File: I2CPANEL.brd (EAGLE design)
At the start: 54 x 83 mm, 47 parts, among them IC1 ATMEGA32U4-QFN

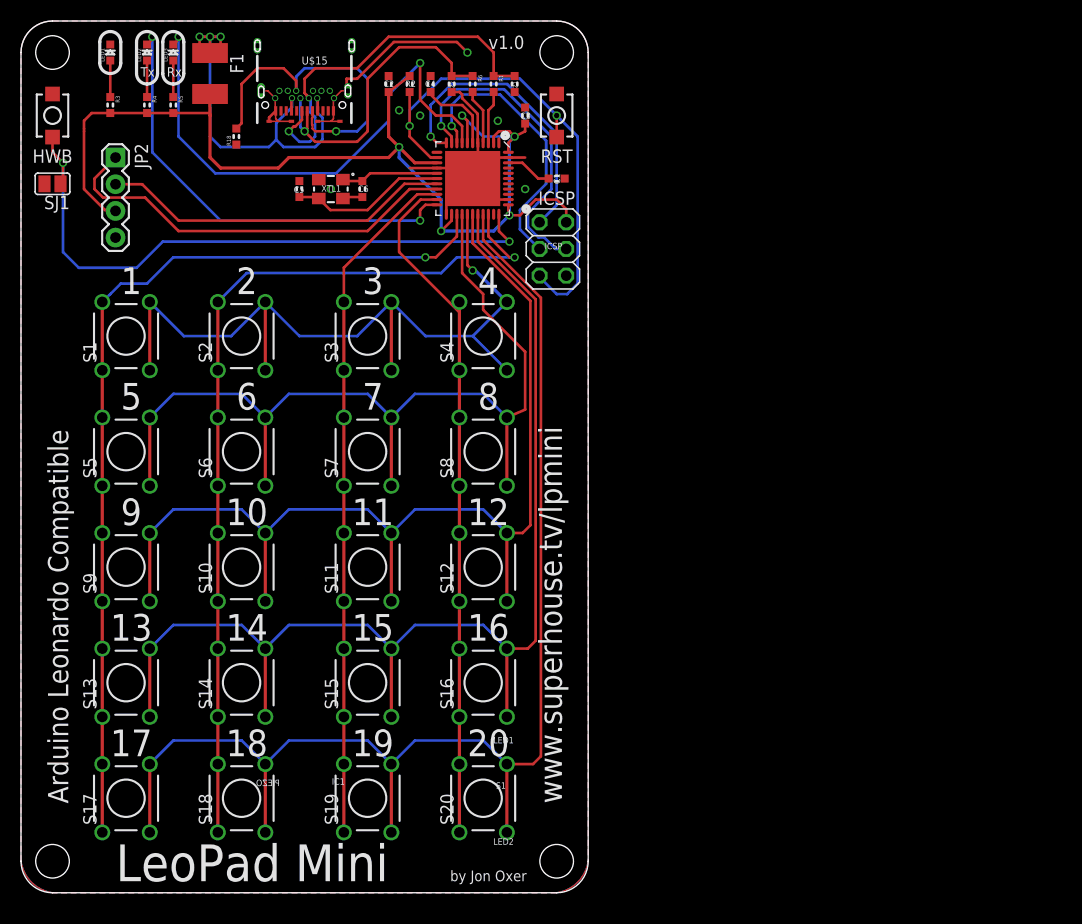
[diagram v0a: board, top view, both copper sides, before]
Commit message: Schematic and routing for v1.0 release
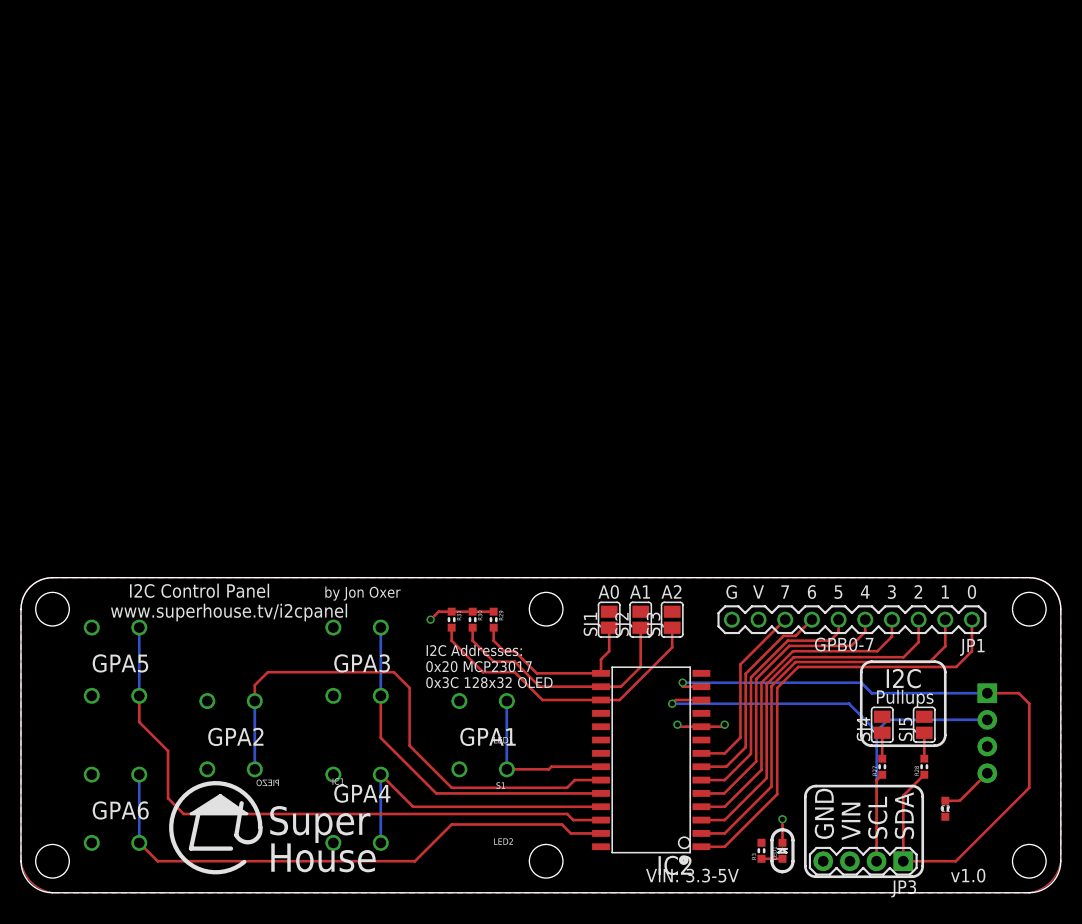
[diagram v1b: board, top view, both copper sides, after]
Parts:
- removed C1: 100nF 0603, freetronics-master-v1.1:0603
- removed C3, C4: 1uF 0603, freetronics-master-v1.1:0603
- removed C5, C6: 15pF 0603, freetronics-master-v1.1:0603
- removed F1: 500mA PTC 1812, rcl:L1812
- removed IC1: ATMEGA32U4-QFN, freetronics-jon:QFN-44N
- removed ICSP: ICSP, pinhead:2X03
- removed LED2: RED, freetronics-jon:LED-0603
- removed LED3: GREEN, freetronics-jon:LED-0603
- removed R1, R6: 22R, freetronics-jon:0603
- removed R18: 5.1K, freetronics-original:0603
- removed R2: 10K 0603, freetronics-master-v1.1:0603
- removed R4, R5: 1K, freetronics-jon:0603
- removed S10: 10, freetronics-original:TACTILE-PTH
- removed S11: 11, freetronics-original:TACTILE-PTH
- removed S12: 12, freetronics-original:TACTILE-PTH
- removed S13: 13, freetronics-original:TACTILE-PTH
- removed S14: 14, freetronics-original:TACTILE-PTH
- removed S15: 15, freetronics-original:TACTILE-PTH
- removed S16: 16, freetronics-original:TACTILE-PTH
- removed S17: 17, freetronics-original:TACTILE-PTH
- removed S18: 18, freetronics-original:TACTILE-PTH
- removed S19: 19, freetronics-original:TACTILE-PTH
- removed S20: 20, freetronics-original:TACTILE-PTH
- removed S21: RESET, freetronics-jon:TACTILE_SWITCH_SMD_2PIN_TINY
- removed S22: HWB, freetronics-jon:TACTILE_SWITCH_SMD_2PIN_TINY
- removed S7: 7, freetronics-original:TACTILE-PTH
- removed S8: 8, freetronics-original:TACTILE-PTH
- removed S9: 9, freetronics-original:TACTILE-PTH
- removed U$15: USB-C, freetronics-jon:USB-C-U52A
- removed XTL1: 16MHz, freetronics-jon:CRYSTAL-SMD-3X2
- removed Z1, Z2: PGB1010603, freetronics-master-v1.1:0603
- added IC2: MCP23017SO, microchip:SO28W
- added JP1: M100.1, freetronics-original:1X10
- added JP3: OLED, freetronics-jon:1X04
- added R27, R28: 4K7, freetronics-master-v1:0603
- added R29, R30, R31: 10K, freetronics-master-v1:0603
- added SJ2, SJ3, SJ4, SJ5: (no value), freetronics-jon:SJ
- C2: value 100nF 0603 -> 1uF
- SJ1: value HWB -> (none)
- moved LED1 99.4 mm to (72.5, 4.00)
- moved JP2 97.4 mm to (92.0, 19.0), flipped to the bottom
- moved R3 94.3 mm to (70.5, 4.00), turned to 90 degrees
- moved C2 87.0 mm to (88.0, 8.00)
- moved SJ1 67.3 mm to (56.0, 26.0), turned to 90 degrees
- moved S1 51.0 mm to (44.0, 15.0), flipped to the bottom
- moved S4 46.6 mm to (32.0, 8.00), flipped to the bottom
- moved S2 38.0 mm to (20.0, 15.0), flipped to the bottom
- moved S6 36.1 mm to (9.00, 8.00), flipped to the bottom
- moved S3 31.0 mm to (32.0, 22.0), flipped to the bottom
- moved S5 20.0 mm to (9.00, 22.0), flipped to the bottom
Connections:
- removed net 3V3: C4.2, IC1.6
- removed net 5V: C2.1, C3.1, F1.2, IC1.14, IC1.2, IC1.24, IC1.34, IC1.44, IC1.7, ICSP.2, JP2.3, R2.2, R3.2, R4.2, R5.2
- removed net A0: IC1.36
- removed net A1: IC1.37
- removed net A2: IC1.38
- removed net A3: IC1.39
- removed net A4: IC1.40
- removed net A5: IC1.41
- removed net AREF: C1.1, IC1.42
- removed net COL0: IC1.25, S1.1, S1.2, S13.1, S13.2, S17.1, S17.2, S5.1, S5.2, S9.1, S9.2
- removed net COL1: IC1.31, S10.1, S10.2, S14.1, S14.2, S18.1, S18.2, S2.1, S2.2, S6.1, S6.2
- removed net COL2: IC1.20, S11.1, S11.2, S15.1, S15.2, S19.1, S19.2, S3.1, S3.2, S7.1, S7.2
- removed net COL3: IC1.21, S12.1, S12.2, S16.1, S16.2, S20.1, S20.2, S4.1, S4.2, S8.1, S8.2
- removed net D+: R6.1, U$15.A6, U$15.B6, Z2.2
- removed net D-: R1.1, U$15.A7, U$15.B7, Z1.2
- removed net D11: IC1.12
- removed net D13: IC1.32
- removed net D2_SDA: IC1.19, JP2.1
- removed net D3_SCL: IC1.18, JP2.2
- removed net D7_AIN0: IC1.1
- removed net HWB: IC1.33, S22.1, SJ1.1
- removed net MISO: IC1.11, ICSP.1
- removed net MOSI: IC1.10, ICSP.4
- removed net N$11: C5.2, IC1.17, XTL1.3
- removed net N$12: C6.2, IC1.16, XTL1.1
- removed net N$67: R18.2, U$15.A5, U$15.B5
- removed net RD+: IC1.4, R6.2
- removed net RD-: IC1.3, R1.2
- removed net RESET: IC1.13, ICSP.5, R2.1, S21.2
- removed net ROW0: IC1.27, S1.3, S1.4, S2.3, S2.4, S3.3, S3.4, S4.3, S4.4
- removed net ROW1: IC1.26, S5.3, S5.4, S6.3, S6.4, S7.3, S7.4, S8.3, S8.4
- removed net ROW2: IC1.28, S10.3, S10.4, S11.3, S11.4, S12.3, S12.4, S9.3, S9.4
- removed net ROW3: IC1.29, S13.3, S13.4, S14.3, S14.4, S15.3, S15.4, S16.3, S16.4
- removed net ROW4: IC1.30, S17.3, S17.4, S18.3, S18.4, S19.3, S19.4, S20.3, S20.4
- removed net RXLED_SS: IC1.8, LED3.C
- removed net SCK: IC1.9, ICSP.3
- removed net TX_LED: IC1.22, LED2.C
- removed net USB+: F1.1, U$15.A4, U$15.A9, U$15.B4, U$15.B9
- new net ADDR0: IC2.15, R29.2, SJ1.1
- new net ADDR1: IC2.16, R30.2, SJ2.1
- new net ADDR2: IC2.17, R31.2, SJ3.1
- new net GPA1: IC2.22, S1.1, S1.2
- new net GPA2: IC2.23, S2.1, S2.2
- new net GPA3: IC2.24, S3.1, S3.2
- new net GPA4: IC2.25, S4.1, S4.2
- new net GPA5: IC2.26, S5.1, S5.2
- new net GPA6: IC2.27, S6.1, S6.2
- new net N$1: IC2.1, JP1.1
- new net N$2: IC2.2, JP1.2
- new net N$3: IC2.3, JP1.3
- new net N$4: IC2.4, JP1.4
- new net N$42: R27.2, SJ4.1
- new net N$43: R28.2, SJ5.1
- new net N$5: IC2.5, JP1.5
- new net N$9: IC2.8, JP1.8
- new net SCL: IC2.12, JP2.2, JP3.2, R27.1
- new net SDA: IC2.13, JP2.1, JP3.1, R28.1
- new net VCC: C2.1, IC2.18, IC2.9, JP1.9, JP2.3, JP3.3, R3.2, SJ1.2, SJ2.2, SJ3.2, SJ4.2, SJ5.2
- net GND: now also IC2.10, JP1.10, JP3.4, R29.1, R30.1, R31.1, S1.3, S1.4, S2.3, S2.4, S3.3, S3.4, S4.3, S4.4, S5.3, S5.4, S6.3, S6.4; no longer C1.2, C3.2, C4.1, C5.1, C6.1, IC1.15, IC1.23, IC1.35, IC1.43, IC1.5, IC1.TGND, ICSP.6, R18.1, S21.1, S22.2, SJ1.2, U$15.A1, U$15.A12, U$15.B1, U$15.B12, U$15.CASE1, U$15.CASE2, U$15.CASE3, U$15.CASE4, U$15.FIX1, U$15.FIX2, U$15.FIX3, U$15.FIX4, XTL1.2, XTL1.4, Z1.1, Z2.1
- net N$7: now also IC2.6, JP1.6; no longer LED2.A, R4.1
- net N$8: now also IC2.7, JP1.7; no longer LED3.A, R5.1
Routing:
- net ROW4: track 123.0 -> 0.00 mm
- net ROW3: track 111.5 -> 0.00 mm
- net 5V: track 111.1 -> 0.00 mm, vias 5 -> 0
- net ROW2: track 100.0 -> 0.00 mm
- net COL0: track 88.9 -> 0.00 mm, vias 1 -> 0
- net ROW1: track 88.6 -> 0.00 mm
- net COL1: track 86.0 -> 0.00 mm, vias 1 -> 0
- net ROW0: track 76.2 -> 0.00 mm, vias 1 -> 0
- net SDA: track 0.00 -> 68.0 mm, vias 0 -> 1
- net COL3: track 67.0 -> 0.00 mm
- net COL2: track 65.5 -> 0.00 mm
- net HWB: track 60.6 -> 0.00 mm, vias 2 -> 0
- net GPA5: track 0.00 -> 59.5 mm
- net SCL: track 0.00 -> 55.3 mm, vias 0 -> 1
- net GPA6: track 0.00 -> 53.0 mm
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- added copper zone on layer 1, net VCC
- removed copper zone on layer 1, net GND
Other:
- board size 54 x 83 mm -> 99 x 30 mm
- board text added: "0"
- board text added: "A0"
- board text added: "A1"
- board text added: "A2"
- board text added: "Copyright 2019 SuperHouse Automation Pty Ltd Released under the TAPR Open Hardware License www.tapr.org/OHL"
- board text added: "G"
- board text added: "GPA1"
- board text added: "GPA2"
- board text added: "GPA3"
- board text added: "GPA4"
- board text added: "GPA5"
- board text added: "GPA6"
- board text added: "GPB0-7"
- board text added: "I2C"
- board text added: "I2C Addresses: 0x20 MCP23017 0x3C 128x32 OLED"
- board text added: "I2C Control Panel"
- board text added: "Pullups"
- board text added: "SCL"
- board text added: "SDA"
- board text added: "V"
- board text added: "VIN"
- board text added: "VIN: 3.3-5V"
- board text added: "www.superhouse.tv/i2cpanel"
- board text removed: "10"
- board text removed: "11"
- board text removed: "12"
- board text removed: "13"
- board text removed: "14"
- board text removed: "15"
- board text removed: "16"
- board text removed: "17"
- board text removed: "18"
- board text removed: "19"
- board text removed: "20"
- board text removed: "8"
- board text removed: "9"
- board text removed: "Arduino Leonardo Compatible"
- board text removed: "Col0: D4 Col1: D5 Col2: D0 Col3: D1"
- board text removed: "Copyright 2018 SuperHouse Automation Pty Ltd Released under the TAPR Open Hardware License www.tapr.org/OHL"
- board text removed: "HWB"
- board text removed: "ICSP"
- board text removed: "LeoPad Mini"
- board text removed: "RST"
- board text removed: "Row0: D6 Row1: D12 Row2: D8 Row3: D9 Row4: D10"
- board text removed: "Rx"
- board text removed: "Tx"
- board text removed: "USB-C"
- board text removed: "www.superhouse.tv/lpmini"
